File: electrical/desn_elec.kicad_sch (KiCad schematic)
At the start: 8 parts, among them J1 LOGITECH F310, M1 ESC_PWM, M2 ESC_PWM, M3 ESC_PWM, U1 ESP32-S3-Zero, U2 LM2596S-MOD, U3 MPU-6050-MOD

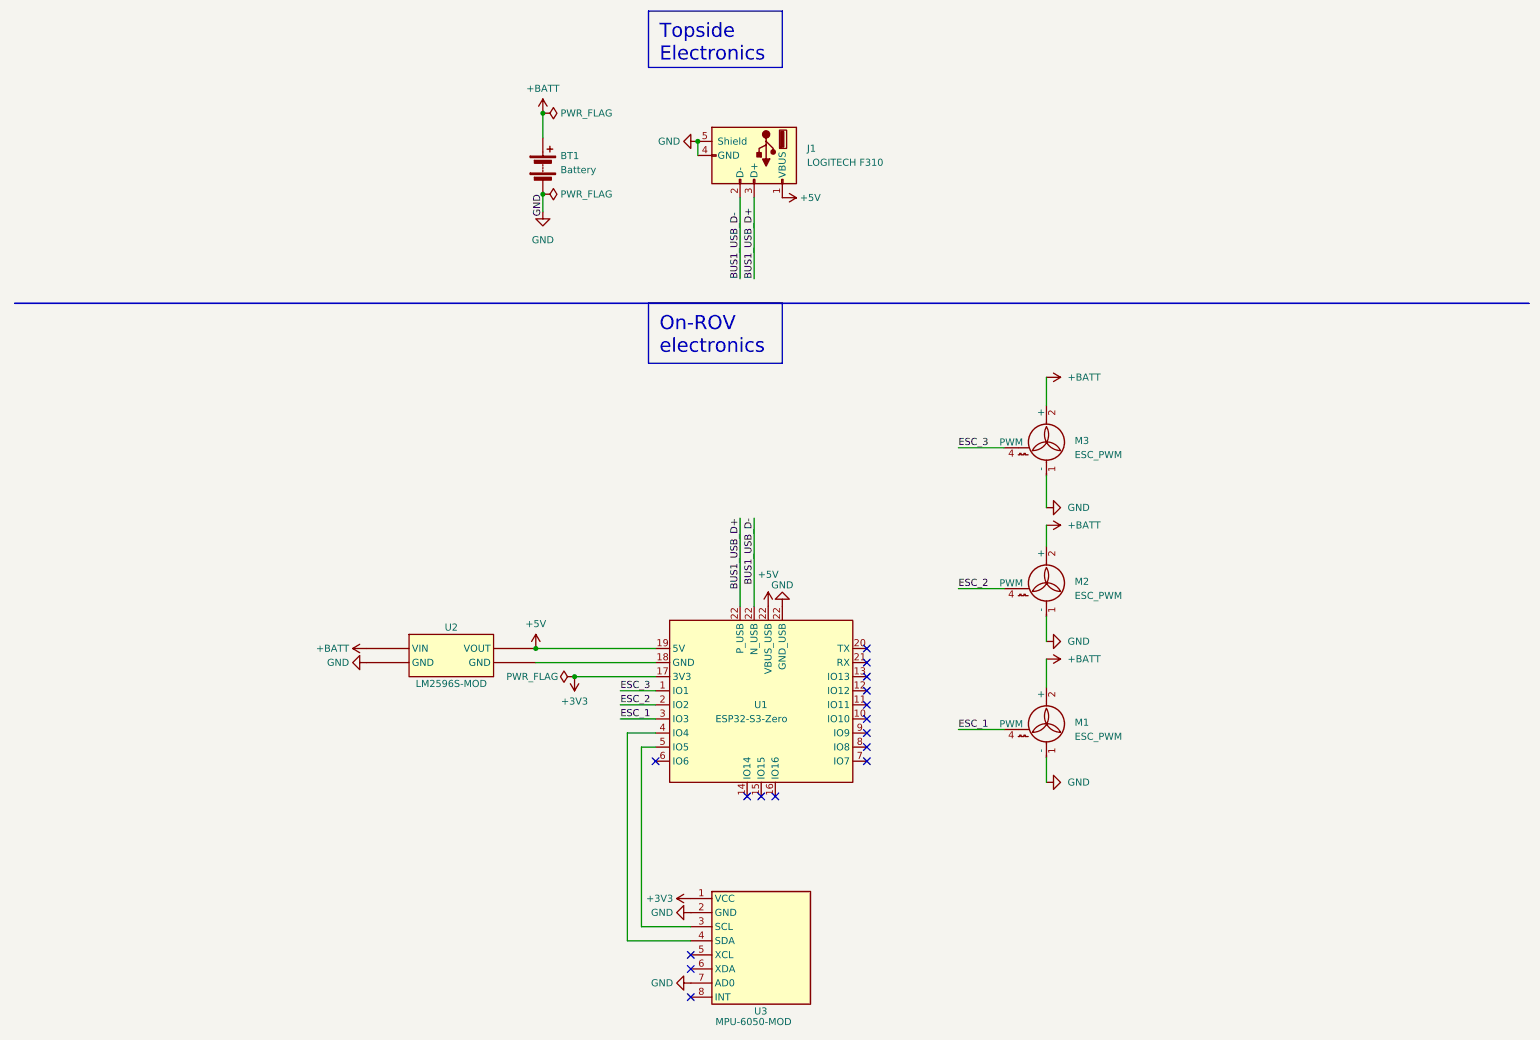
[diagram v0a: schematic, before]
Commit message: updates
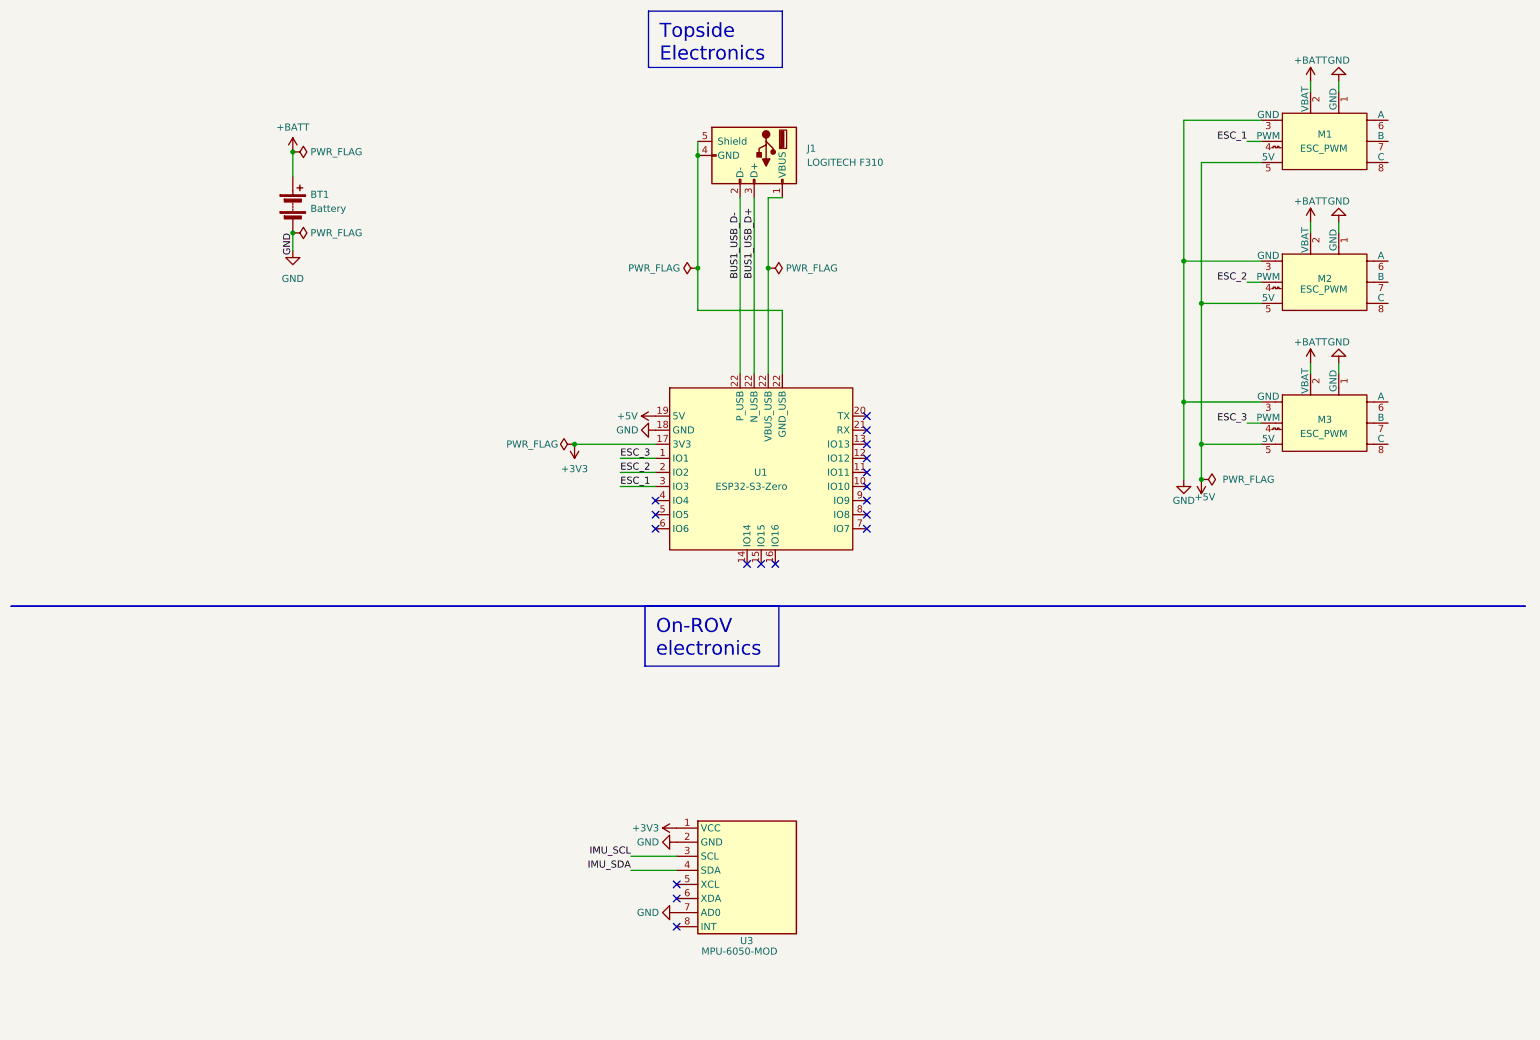
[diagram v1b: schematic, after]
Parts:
- removed U2: LM2596S-MOD, symbol PROJECT_SYM:LM2596S-MOD
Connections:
- net +5V: now also M1.5 (5V), M2.5 (5V), M3.5 (5V); no longer J1.1 (VBUS), U1.22 (VBUS_USB)
- net GND: now also M1.3 (GND), M2.3 (GND), M3.3 (GND), U1.18 (GND); no longer J1.4 (GND), J1.5 (Shield), U1.22 (VBUS_USB)
- net at U1.4 (IO4): no longer U3.4 (SDA)
- net at U1.5 (IO5): no longer U3.3 (SCL)
- new net: J1.1 (VBUS), U1.22 (VBUS_USB)
- new net: J1.4 (GND), J1.5 (Shield), U1.22 (VBUS_USB)
- new net IMU_SCL: U3.3 (SCL)
- new net IMU_SDA: U3.4 (SDA)
- no-connect marks 16 -> 18
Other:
- moved on the sheet: BT1, U1, U3
